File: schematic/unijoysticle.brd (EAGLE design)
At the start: 69.5 x 69.8 mm, 8 parts, among them CN1 DC JACK, IC1 4066N, IC2 4066N, IC3 4066N, X1 DSUB 9, X2 DSUB 9

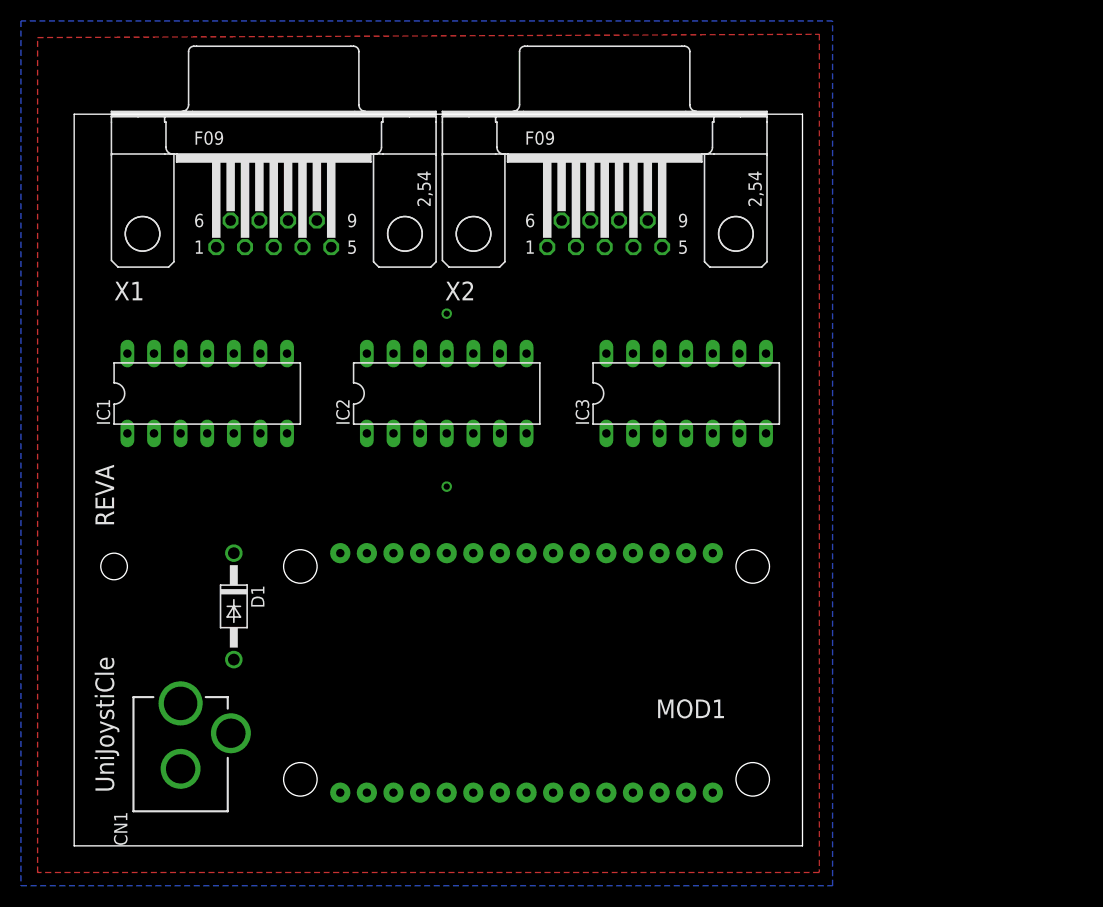
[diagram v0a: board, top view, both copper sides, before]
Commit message: fix: new design
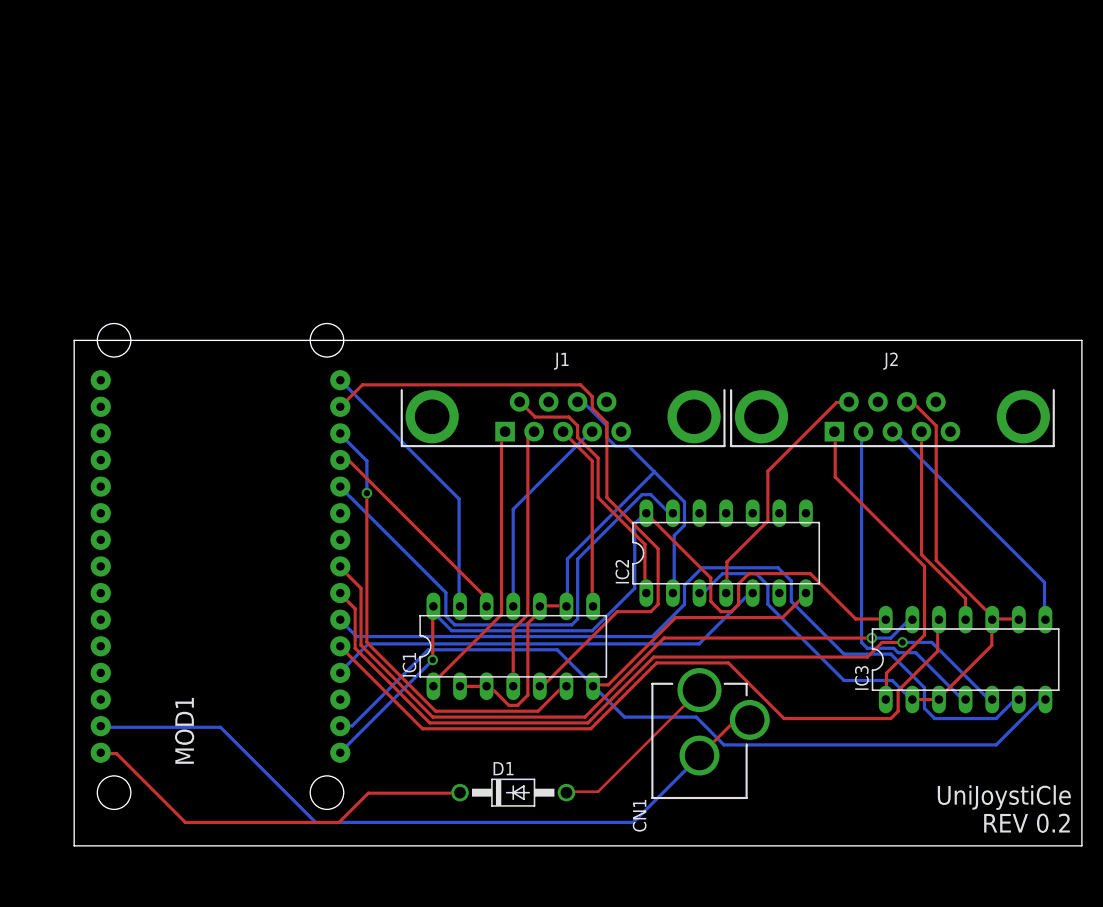
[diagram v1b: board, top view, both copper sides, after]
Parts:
- removed X1, X2: DSUB 9, con-subd:F09H
- added J1, J2: DB9, SparkFun-Connectors:DB9
- moved CN1 49.5 mm to (59.7, 1.27)
- moved IC1 37.9 mm to (41.9, 19.1)
- moved IC3 36.8 mm to (85.1, 17.8)
- moved D1 32.1 mm to (41.9, 5.08), turned to 0 degrees
- moved MOD1 30.9 mm to (14.0, 26.7), turned to 0 degrees
- moved IC2 30.7 mm to (62.2, 27.9)
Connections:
- net N$10: now also J1.2; no longer X1.2
- net N$11: now also J1.3; no longer X1.3
- net N$12: now also J1.4; no longer X1.4
- net N$13: now also J2.1; no longer X2.1
- net N$14: now also J2.2; no longer X2.2
- net N$15: now also J2.3; no longer X2.3
- net N$16: now also J2.4; no longer X2.4
- net N$17: now also J1.8; no longer X1.8
- net N$18: now also J2.8; no longer X2.8
- net N$21: now also J1.6; no longer X1.6
- net N$22: now also J2.6; no longer X2.6
- net N$9: now also J1.1; no longer X1.1
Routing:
- net GND: track 0.00 -> 100.0 mm
- net VCC: track 0.00 -> 80.0 mm, vias 0 -> 1
- net N$7: track 0.00 -> 78.2 mm
- net N$6: track 0.00 -> 75.1 mm, vias 0 -> 1
- net N$8: track 0.00 -> 72.0 mm
- net 3.3V: track 0.00 -> 69.8 mm
- net N$5: track 0.00 -> 67.7 mm, vias 0 -> 1
- net N$18: track 0.00 -> 66.5 mm
- net N$2: track 0.00 -> 62.4 mm
- net N$17: track 0.00 -> 59.5 mm
- net N$19: track 0.00 -> 47.8 mm
- net N$3: track 0.00 -> 43.8 mm, vias 0 -> 1
- net N$20: track 0.00 -> 42.6 mm
- net 5V: track 0.00 -> 38.2 mm
- net N$14: track 0.00 -> 32.4 mm
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- removed copper zone on layer 1, net GND
- removed copper zone on layer 16, net GND
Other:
- board size 69.5 x 69.8 mm -> 96.2 x 48.2 mm
- board text added: "UniJoystiCle REV 0.2"
- board text added: "http://retro.moe"
- board text removed: "REVA"
- board text removed: "UniJoystiCle"
